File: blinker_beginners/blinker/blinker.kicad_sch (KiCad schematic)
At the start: 8 parts, among them SW1 SW_MEC_5E, U1 NE555P

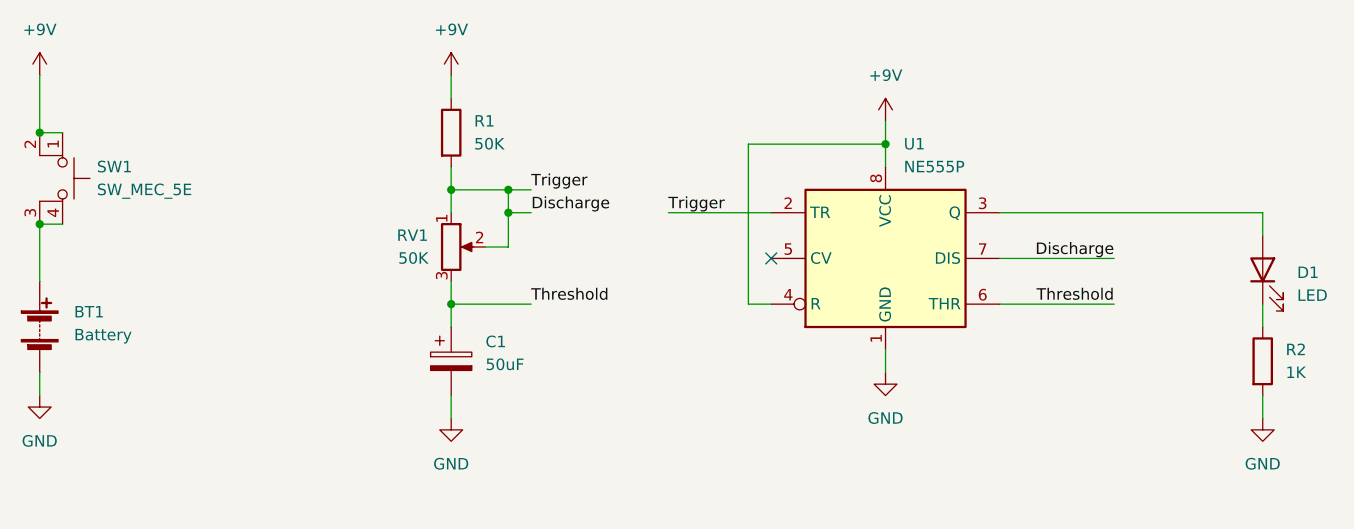
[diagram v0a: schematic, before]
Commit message: fixes
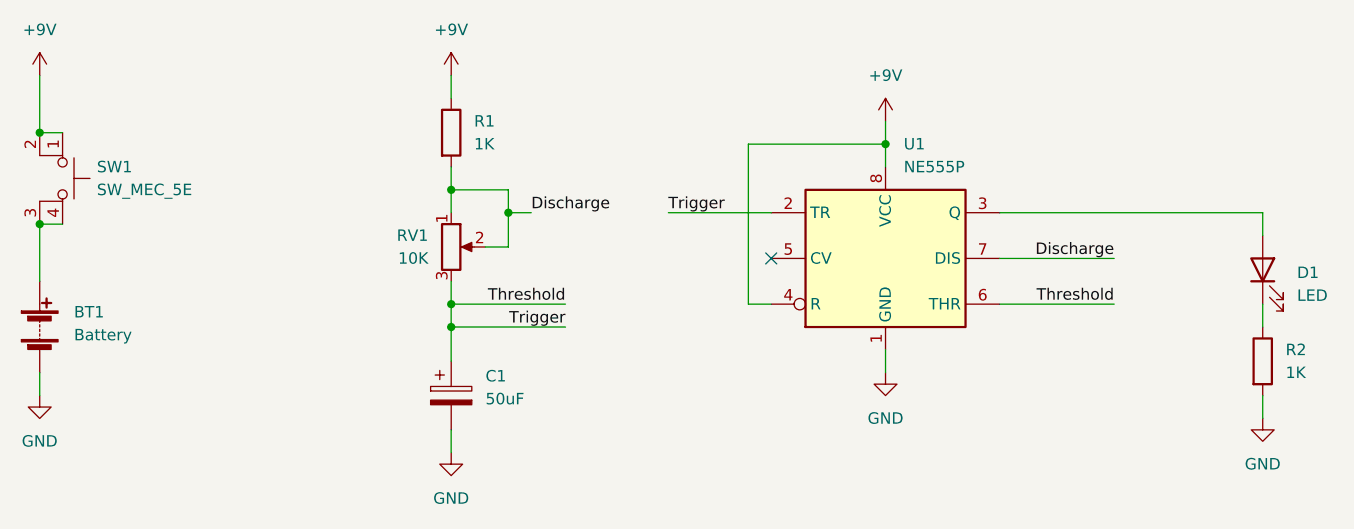
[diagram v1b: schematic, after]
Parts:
- R1: value 50K -> 1K
- RV1: value 50K -> 10K
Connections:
- net Discharge: no longer U1.2 (TR)
- net Threshold: now also U1.2 (TR)
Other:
- moved on the sheet: C1
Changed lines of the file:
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@@
   (junction (at 25.4 44.45) (diameter 0) (color 0 0 0 0)
   )
+  (junction (at 71.12 55.88) (diameter 0) (color 0 0 0 0)
+  )
   (junction (at 25.4 34.29) (diameter 0) (color 0 0 0 0)
   )
@@
   )
   (junction (at 119.38 35.56) (diameter 0) (color 0 0 0 0)
-  )
-  (junction (at 77.47 40.64) (diameter 0) (color 0 0 0 0)
   )
   (no_connect (at 106.68 48.26))
@@
     (stroke (width 0) (type default) (color 0 0 0 0))
   )
-  (wire (pts (xy 71.12 53.34) (xy 80.01 53.34))
+  (wire (pts (xy 71.12 53.34) (xy 83.82 53.34))
     (stroke (width 0) (type default) (color 0 0 0 0))
   )
@@
     (stroke (width 0) (type default) (color 0 0 0 0))
   )
-  (wire (pts (xy 77.47 40.64) (xy 80.01 40.64))
+  (wire (pts (xy 71.12 55.88) (xy 71.12 59.69))
     (stroke (width 0) (type default) (color 0 0 0 0))
   )
@@
     (stroke (width 0) (type default) (color 0 0 0 0))
   )
-  (wire (pts (xy 71.12 63.5) (xy 71.12 66.04))
+  (wire (pts (xy 71.12 67.31) (xy 71.12 69.85))
     (stroke (width 0) (type default) (color 0 0 0 0))
   )
@@
     (stroke (width 0) (type default) (color 0 0 0 0))
   )
+  (wire (pts (xy 71.12 55.88) (xy 83.82 55.88))
+    (stroke (width 0) (type default) (color 0 0 0 0))
+  )
   (wire (pts (xy 71.12 50.8) (xy 71.12 53.34))
     (stroke (width 0) (type default) (color 0 0 0 0))
@@
     (stroke (width 0) (type default) (color 0 0 0 0))
   )
-  (label "Threshold" (at 80.01 53.34 0)
-    (effects (font (size 1.27 1.27)) (justify left bottom))
+  (label "Threshold" (at 83.82 53.34 180)
+    (effects (font (size 1.27 1.27)) (justify right bottom))
   )
   (label "Discharge" (at 144.78 48.26 180)
@@
     (effects (font (size 1.27 1.27)) (justify left bottom))
   )
-  (label "Trigger" (at 80.01 40.64 0)
-    (effects (font (size 1.27 1.27)) (justify left bottom))
+  (label "Trigger" (at 83.82 55.88 180)
+    (effects (font (size 1.27 1.27)) (justify right bottom))
   )
   (label "Threshold" (at 144.78 53.34 180)
@@
       (effects (font (size 1.27 1.27)) (justify left))
     )
-    (property "Value" "50K" (id 1) (at 73.66 35.5599 0)
+    (property "Value" "1K" (id 1) (at 73.66 35.5599 0)
       (effects (font (size 1.27 1.27)) (justify left))
     )
@@
     (pin "4")
   )
-  (symbol (lib_id "Device:C_Polarized") (at 71.12 59.69 0) (unit 1)
-    (in_bom yes) (on_board yes) (fields_autoplaced)
-    (property "Reference" "C1" (id 0) (at 74.93 57.5309 0)
-      (effects (font (size 1.27 1.27)) (justify left))
-    )
-    (property "Value" "50uF" (id 1) (at 74.93 60.0709 0)
-      (effects (font (size 1.27 1.27)) (justify left))
-    )
-    (property "Footprint" "Capacitor_THT:CP_Radial_D5.0mm_P2.00mm" (id 2) (at 72.0852 63.5 0)
-      (effects (font (size 1.27 1.27)) hide)
-    )
-    (property "Datasheet" "~" (id 3) (at 71.12 59.69 0)
+  (symbol (lib_id "Device:C_Polarized") (at 71.12 63.5 0) (unit 1)
+    (in_bom yes) (on_board yes) (fields_autoplaced)
+    (property "Reference" "C1" (id 0) (at 74.93 61.3409 0)
+      (effects (font (size 1.27 1.27)) (justify left))
+    )
+    (property "Value" "50uF" (id 1) (at 74.93 63.8809 0)
+      (effects (font (size 1.27 1.27)) (justify left))
+    )
+    (property "Footprint" "Capacitor_THT:CP_Radial_D5.0mm_P2.00mm" (id 2) (at 72.0852 67.31 0)
+      (effects (font (size 1.27 1.27)) hide)
+    )
+    (property "Datasheet" "~" (id 3) (at 71.12 63.5 0)
       (effects (font (size 1.27 1.27)) hide)
     )
@@
       (effects (font (size 1.27 1.27)) (justify right))
     )
-    (property "Value" "50K" (id 1) (at 68.58 48.2599 0)
+    (property "Value" "10K" (id 1) (at 68.58 48.2599 0)
       (effects (font (size 1.27 1.27)) (justify right))
     )
@@
     (pin "1")
   )
-  (symbol (lib_id "power:GND") (at 71.12 66.04 0) (unit 1)
-    (in_bom yes) (on_board yes) (fields_autoplaced)
-    (property "Reference" "#PWR04" (id 0) (at 71.12 72.39 0)
-      (effects (font (size 1.27 1.27)) hide)
-    )
-    (property "Value" "GND" (id 1) (at 71.12 71.12 0))
-    (property "Footprint" "" (id 2) (at 71.12 66.04 0)
-      (effects (font (size 1.27 1.27)) hide)
-    )
-    (property "Datasheet" "" (id 3) (at 71.12 66.04 0)
+  (symbol (lib_id "power:GND") (at 71.12 69.85 0) (unit 1)
+    (in_bom yes) (on_board yes) (fields_autoplaced)
+    (property "Reference" "#PWR04" (id 0) (at 71.12 76.2 0)
+      (effects (font (size 1.27 1.27)) hide)
+    )
+    (property "Value" "GND" (id 1) (at 71.12 74.93 0))
+    (property "Footprint" "" (id 2) (at 71.12 69.85 0)
+      (effects (font (size 1.27 1.27)) hide)
+    )
+    (property "Datasheet" "" (id 3) (at 71.12 69.85 0)
       (effects (font (size 1.27 1.27)) hide)
     )
@@
     )
     (path "/47484446-e64c-4a82-88af-15de92cf6ad4"
-      (reference "R1") (unit 1) (value "50K") (footprint "Resistor_THT:R_Axial_DIN0207_L6.3mm_D2.5mm_P7.62mm_Horizontal")
+      (reference "R1") (unit 1) (value "1K") (footprint "Resistor_THT:R_Axial_DIN0207_L6.3mm_D2.5mm_P7.62mm_Horizontal")
     )
     (path "/c7db4903-f95a-49f5-bcce-c52f0ca8defc"
@@
     )
     (path "/b5cea0b5-192f-476b-a3c8-0c26e2231699"
-      (reference "RV1") (unit 1) (value "50K") (footprint "Potentiometer_THT:Potentiometer_Piher_PT-15-V02_Vertical")
+      (reference "RV1") (unit 1) (value "10K") (footprint "Potentiometer_THT:Potentiometer_Piher_PT-15-V02_Vertical")
     )
     (path "/5fe24dd1-2949-489e-a84c-0ddc068c606c"

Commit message: pcb design for board rev 1
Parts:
- U1: footprint timer_footprints:DIP-8_W7.62mm_InvertedDualRow -> Package_DIP:DIP-8_W7.62mm
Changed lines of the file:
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@@
       (effects (font (size 1.27 1.27)) (justify left))
     )
-    (property "Footprint" "timer_footprints:DIP-8_W7.62mm_InvertedDualRow" (id 2) (at 135.89 58.42 0)
+    (property "Footprint" "Package_DIP:DIP-8_W7.62mm" (id 2) (at 135.89 58.42 0)
       (effects (font (size 1.27 1.27)) hide)
     )
@@
     )
     (path "/a4541b62-7a39-4707-9c6f-80dce1be9cee"
-      (reference "U1") (unit 1) (value "NE555P") (footprint "timer_footprints:DIP-8_W7.62mm_InvertedDualRow")
+      (reference "U1") (unit 1) (value "NE555P") (footprint "Package_DIP:DIP-8_W7.62mm")
     )
   )
